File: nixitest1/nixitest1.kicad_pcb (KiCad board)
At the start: 2 copper layers, 22 x 38 mm, 32 parts, among them J1 MSYS, Q1 60V 3A, Q10 HVN, Q11 HVN, Q12 HVN, Q13 HVN, Q2 HVN, Q3 HVN, Q4 HVN, Q5 HVN, Q6 HVN, Q7 HVN, Q8 HVN, Q9 HVN, T1 Flyback-ATB3225, U1 CH32V003F4U6, U2 IN12-NIXIETUBE

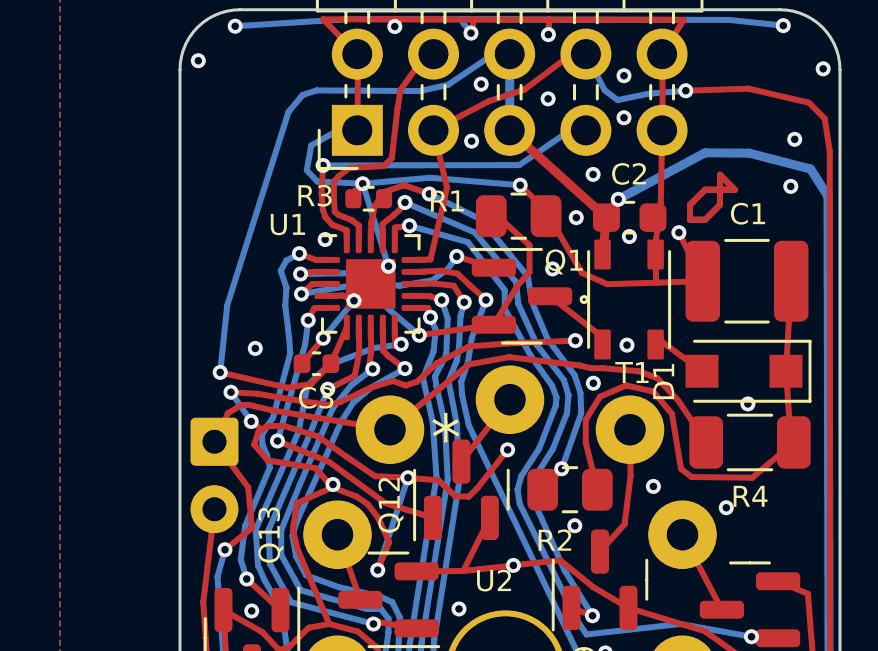
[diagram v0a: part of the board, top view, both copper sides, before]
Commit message: Update board design
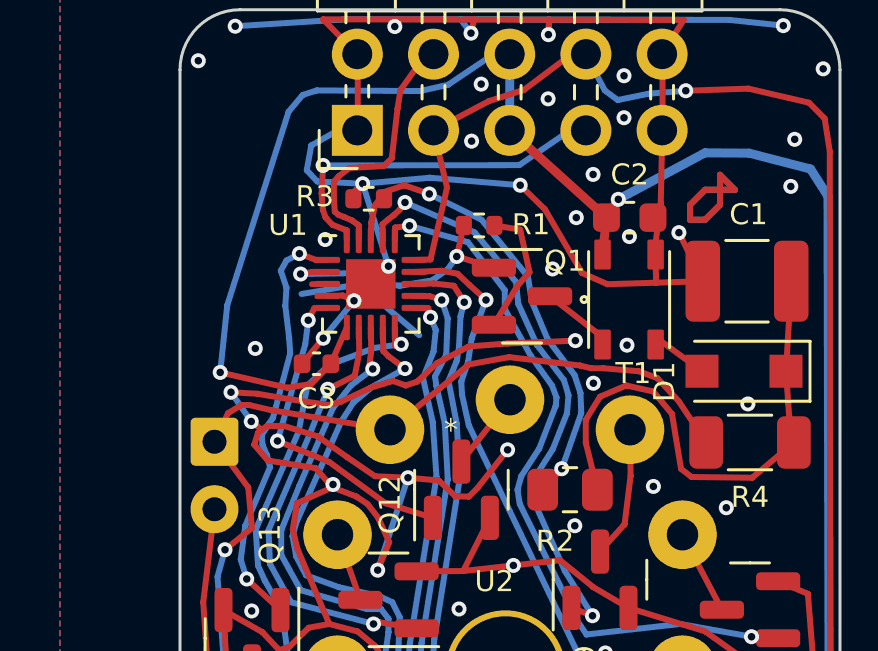
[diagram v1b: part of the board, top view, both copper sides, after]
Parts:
- R1: value 500mΩ -> 10k; footprint Resistor_SMD:R_0805_2012Metric -> Resistor_SMD:R_0402_1005Metric
- moved R1 1.36 mm to (89.0, 65.2), turned to 180 degrees
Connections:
- Q1 pad 2: HVIMON -> GND
- R1 pad 1: HVIMON -> GND
- R1 pad 2: GND -> HVCTL
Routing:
- net HVIMON: track 12.9 -> 0.51 mm, vias 2 -> 0
- net GND: track 172.8 -> 181.8 mm
- net HVCTL: track 7.85 -> 8.91 mm
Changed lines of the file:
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@@
     )
   )
-  (footprint "Resistor_SMD:R_0805_2012Metric" (layer "F.Cu")
-    (at 90.29 64.88)
-    (descr "Resistor SMD 0805 (2012 Metric), square (rectangular) end terminal, IPC_7351 nominal, (Body size source: IPC-SM-782 page 72, https://www.pcb-3d.com/wordpress/wp-content/uploads/ipc-sm-782a_amendment_1_and_2.pdf), generated with kicad-footprint-generator")
+  (footprint "Resistor_SMD:R_0402_1005Metric" (layer "F.Cu")
+    (at 88.97 65.19 180)
+    (descr "Resistor SMD 0402 (1005 Metric), square (rectangular) end terminal, IPC_7351 nominal, (Body size source: IPC-SM-782 page 72, https://www.pcb-3d.com/wordpress/wp-content/uploads/ipc-sm-782a_amendment_1_and_2.pdf), generated with kicad-footprint-generator")
     (tags "resistor")
-    (property "LCSC" "C327217")
-    (property "Sheetfile" "nixitest1.kicad_sch")
-    (property "Sheetname" "")
-    (attr smd)
-    (fp_text reference "R1" (at -2.38 -0.48 unlocked) (layer "F.SilkS")
-      (effects (font (size 0.7 0.7) (thickness 0.1)))
-    )
-    (fp_text value "500mΩ" (at 0 1.65 unlocked) (layer "F.Fab")
+    (property "LCSC" "C25744")
+    (property "Sheetfile" "nixitest1.kicad_sch")
+    (property "Sheetname" "")
+    (attr smd)
+    (fp_text reference "R1" (at -1.73 0.03 unlocked) (layer "F.SilkS")
+      (effects (font (size 0.7 0.7) (thickness 0.1)))
+    )
+    (fp_text value "10k" (at 0 1.17 unlocked) (layer "F.Fab")
       (effects (font (size 1 1) (thickness 0.15)))
     )
@@
       (effects (font (size 1 1) (thickness 0.15)))
     )
-    (fp_line (start -0.227064 -0.735) (end 0.227064 -0.735) (layer "F.SilkS") (width 0.1))
-    (fp_line (start -0.227064 0.735) (end 0.227064 0.735) (layer "F.SilkS") (width 0.1))
-    (fp_line (start -1.68 0.95) (end -1.68 -0.95) (layer "F.CrtYd") (width 0.05))
-    (fp_line (start -1.68 -0.95) (end 1.68 -0.95) (layer "F.CrtYd") (width 0.05))
-    (fp_line (start 1.68 -0.95) (end 1.68 0.95) (layer "F.CrtYd") (width 0.05))
-    (fp_line (start 1.68 0.95) (end -1.68 0.95) (layer "F.CrtYd") (width 0.05))
-    (fp_line (start -1 0.625) (end -1 -0.625) (layer "F.Fab") (width 0.1))
-    (fp_line (start 1 -0.625) (end 1 0.625) (layer "F.Fab") (width 0.1))
-    (fp_line (start 1 0.625) (end -1 0.625) (layer "F.Fab") (width 0.1))
-    (fp_line (start -1 -0.625) (end 1 -0.625) (layer "F.Fab") (width 0.1))
-    (pad "1" smd roundrect locked (at -0.9125 0) (size 1.025 1.4) (layers "F.Cu" "F.Paste" "F.Mask") (roundrect_rratio 0.243902439)
-      (net 5 "HVIMON") (pintype "passive"))
-    (pad "2" smd roundrect locked (at 0.9125 0) (size 1.025 1.4) (layers "F.Cu" "F.Paste" "F.Mask") (roundrect_rratio 0.243902439)
+    (fp_line (start -0.153641 -0.38) (end 0.153641 -0.38) (layer "F.SilkS") (width 0.1))
+    (fp_line (start -0.153641 0.38) (end 0.153641 0.38) (layer "F.SilkS") (width 0.1))
+    (fp_line (start 0.93 0.47) (end -0.93 0.47) (layer "F.CrtYd") (width 0.05))
+    (fp_line (start 0.93 -0.47) (end 0.93 0.47) (layer "F.CrtYd") (width 0.05))
+    (fp_line (start -0.93 -0.47) (end 0.93 -0.47) (layer "F.CrtYd") (width 0.05))
+    (fp_line (start -0.93 0.47) (end -0.93 -0.47) (layer "F.CrtYd") (width 0.05))
+    (fp_line (start 0.525 0.27) (end -0.525 0.27) (layer "F.Fab") (width 0.1))
+    (fp_line (start 0.525 -0.27) (end 0.525 0.27) (layer "F.Fab") (width 0.1))
+    (fp_line (start -0.525 -0.27) (end 0.525 -0.27) (layer "F.Fab") (width 0.1))
+    (fp_line (start -0.525 0.27) (end -0.525 -0.27) (layer "F.Fab") (width 0.1))
+    (pad "1" smd roundrect (at -0.51 0 180) (size 0.54 0.64) (layers "F.Cu" "F.Paste" "F.Mask") (roundrect_rratio 0.25)
       (net 2 "GND") (pintype "passive"))
-    (model "${KICAD6_3DMODEL_DIR}/Resistor_SMD.3dshapes/R_0805_2012Metric.wrl"
+    (pad "2" smd roundrect (at 0.51 0 180) (size 0.54 0.64) (layers "F.Cu" "F.Paste" "F.Mask") (roundrect_rratio 0.25)
+      (net 4 "HVCTL") (pintype "passive"))
+    (model "${KICAD6_3DMODEL_DIR}/Resistor_SMD.3dshapes/R_0402_1005Metric.wrl"
       (offset (xyz 0 0 0))
       (scale (xyz 1 1 1))
@@
       (net 4 "HVCTL") (pinfunction "G") (pintype "input"))
     (pad "2" smd roundrect (at -0.9375 0.95) (size 1.475 0.6) (layers "F.Cu" "F.Paste" "F.Mask") (roundrect_rratio 0.25)
-      (net 5 "HVIMON") (pinfunction "S") (pintype "passive"))
+      (net 2 "GND") (pinfunction "S") (pintype "passive"))
     (pad "3" smd roundrect (at 0.9375 0) (size 1.475 0.6) (layers "F.Cu" "F.Paste" "F.Mask") (roundrect_rratio 0.25)
       (net 6 "Net-(Q1-Pad3)") (pinfunction "D") (pintype "passive"))
@@
   (footprint "IN12-NIXIE:IN12-NIXIE" (layer "F.Cu")
     (at 90 80)
-    (property "LCSC" "~")
+    (property "LCSC" "")
     (property "Sheetfile" "nixitest1.kicad_sch")
     (property "Sheetname" "")
@@
   (gr_arc (start 99 58) (mid 100.414214 58.585786) (end 101 60) (layer "Edge.Cuts") (width 0.1))
   (gr_text "*" (at 87.42 71.84 -120) (layer "B.SilkS")
-    (effects (font (size 1.5 1.5) (thickness 0.15)) (justify mirror))
+    (effects (font (size 0.7 0.7) (thickness 0.1)) (justify mirror))
   )
   (gr_text "GND" (at 85.26 94.31) (layer "F.SilkS")
@@
   )
   (gr_text "*" (at 88.175 71.75 120) (layer "F.SilkS")
-    (effects (font (size 1.5 1.5) (thickness 0.15)))
+    (effects (font (size 0.7 0.7) (thickness 0.1)))
   )
   (gr_text "PGM" (at 94.81 94.35) (layer "F.SilkS")
@@
   (segment (start 82.6 70.975) (end 83.95 71.175) (width 0.2) (layer "F.Cu") (net 2))
   (segment (start 91.307459 58.332541) (end 88.801628 58.328372) (width 0.2) (layer "F.Cu") (net 2))
+  (segment (start 89.48 65.19) (end 90.34 65.33) (width 0.2) (layer "F.Cu") (net 2))
   (segment (start 87.98 82.51) (end 88.2875 84.99) (width 0.2) (layer "F.Cu") (net 2))
   (segment (start 84.925 78.725) (end 85.525 79.225) (width 0.2) (layer "F.Cu") (net 2))
@@
   (segment (start 81.67 81.33) (end 80.925 80.85) (width 0.2) (layer "F.Cu") (net 2))
   (segment (start 84.79 64.075) (end 85.09 63.8) (width 0.2) (layer "F.Cu") (net 2))
+  (segment (start 90.34 65.33) (end 90.65 66.75) (width 0.2) (layer "F.Cu") (net 2))
   (segment (start 93.25 67.15) (end 94.873855 67.098855) (width 0.2) (layer "F.Cu") (net 2))
+  (segment (start 90.65 66.75) (end 90.25 67.2) (width 0.2) (layer "F.Cu") (net 2))
   (segment (start 90.113482 76.523482) (end 91.67 76.35) (width 0.2) (layer "F.Cu") (net 2))
   (segment (start 93.77 85.88) (end 92.0025 85.74) (width 0.2) (layer "F.Cu") (net 2))
@@
   (segment (start 82.9 74.45) (end 82.76 75.32) (width 0.2) (layer "F.Cu") (net 2))
   (segment (start 82.91 75.96) (end 83.9758 78.4758) (width 0.2) (layer "F.Cu") (net 2))
+  (segment (start 90.25 67.2) (end 89.4625 68.5) (width 0.2) (layer "F.Cu") (net 2))
   (segment (start 97.61 79.51) (end 99.0575 81.02) (width 0.2) (layer "F.Cu") (net 2))
   (segment (start 83.52 73.28) (end 84.08 73.92) (width 0.2) (layer "F.Cu") (net 2))
@@
   (segment (start 91.28 58.83) (end 91.305749 58.325749) (width 0.2) (layer "B.Cu") (net 2))
   (segment (start 83.575 63.725) (end 83.225 63.35) (width 0.2) (layer "B.Cu") (net 2))
+  (segment (start 86.975 68.85) (end 85.1 67.25) (width 0.2) (layer "B.Cu") (net 2))
   (segment (start 87.33 63.6) (end 85.09 63.8) (width 0.2) (layer "B.Cu") (net 2))
   (segment (start 85.09 63.8) (end 83.575 63.725) (width 0.2) (layer "B.Cu") (net 2))
@@
   (segment (start 83.375 62.525) (end 84.925 61.65) (width 0.2) (layer "B.Cu") (net 2))
   (segment (start 85.95 66.55) (end 85.09 63.8) (width 0.2) (layer "B.Cu") (net 2))
+  (segment (start 84.825 67.175) (end 83.05 67.475) (width 0.2) (layer "B.Cu") (net 2))
   (segment (start 80.84 58.55) (end 84.67 58.31) (width 0.2) (layer "B.Cu") (net 2))
+  (segment (start 85.1 67.25) (end 84.825 67.175) (width 0.2) (layer "B.Cu") (net 2))
   (segment (start 83.225 63.35) (end 83.375 62.525) (width 0.2) (layer "B.Cu") (net 2))
   (segment (start 88.351263 58.318737) (end 91.305749 58.325749) (width 0.2) (layer "B.Cu") (net 2))
@@
   (segment (start 88.225 66.225) (end 89.4625 66.6) (width 0.2) (layer "F.Cu") (net 4))
   (segment (start 83.41 66.74) (end 83.02 66.81) (width 0.2) (layer "F.Cu") (net 4))
+  (segment (start 88.225 66.225) (end 88.46 65.19) (width 0.2) (layer "F.Cu") (net 4))
   (segment (start 83.909999 66.74) (end 83.41 66.74) (width 0.2) (layer "F.Cu") (net 4))
   (via (at 88.225 66.225) (size 0.5) (drill 0.25) (layers "F.Cu" "B.Cu") (net 4))
@@
   (segment (start 87.925 66.65) (end 88.225 66.225) (width 0.2) (layer "B.Cu") (net 4))
   (segment (start 85.75 67.125) (end 86.325 67.2) (width 0.2) (layer "B.Cu") (net 4))
-  (segment (start 89.3375 64.65) (end 90.65 65.85) (width 0.2) (layer "F.Cu") (net 5))
   (segment (start 83.909999 67.14) (end 83.4 67.15) (width 0.2) (layer "F.Cu") (net 5))
-  (segment (start 83.4 67.15) (end 83.05 67.475) (width 0.2) (layer "F.Cu") (net 5))
-  (segment (start 90.25 67.2) (end 89.4625 68.5) (width 0.2) (layer "F.Cu") (net 5))
-  (segment (start 86.975 68.85) (end 89.4625 68.5) (width 0.2) (layer "F.Cu") (net 5))
-  (segment (start 90.65 65.85) (end 90.65 66.75) (width 0.2) (layer "F.Cu") (net 5))
-  (segment (start 90.65 66.75) (end 90.25 67.2) (width 0.2) (layer "F.Cu") (net 5))
-  (via (at 83.05 67.475) (size 0.5) (drill 0.25) (layers "F.Cu" "B.Cu") (net 5))
-  (via (at 86.975 68.85) (size 0.5) (drill 0.25) (layers "F.Cu" "B.Cu") (net 5))
-  (segment (start 86.975 68.85) (end 85.1 67.25) (width 0.2) (layer "B.Cu") (net 5))
-  (segment (start 84.825 67.175) (end 83.05 67.475) (width 0.2) (layer "B.Cu") (net 5))
-  (segment (start 85.1 67.25) (end 84.825 67.175) (width 0.2) (layer "B.Cu") (net 5))
   (segment (start 91.3375 67.55) (end 93.065 68.9) (width 0.2) (layer "F.Cu") (net 6))
   (segment (start 85.66 78.42) (end 86.8875 78.62) (width 0.2) (layer "F.Cu") (net 7))
